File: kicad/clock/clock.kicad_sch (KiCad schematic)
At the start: 6 parts

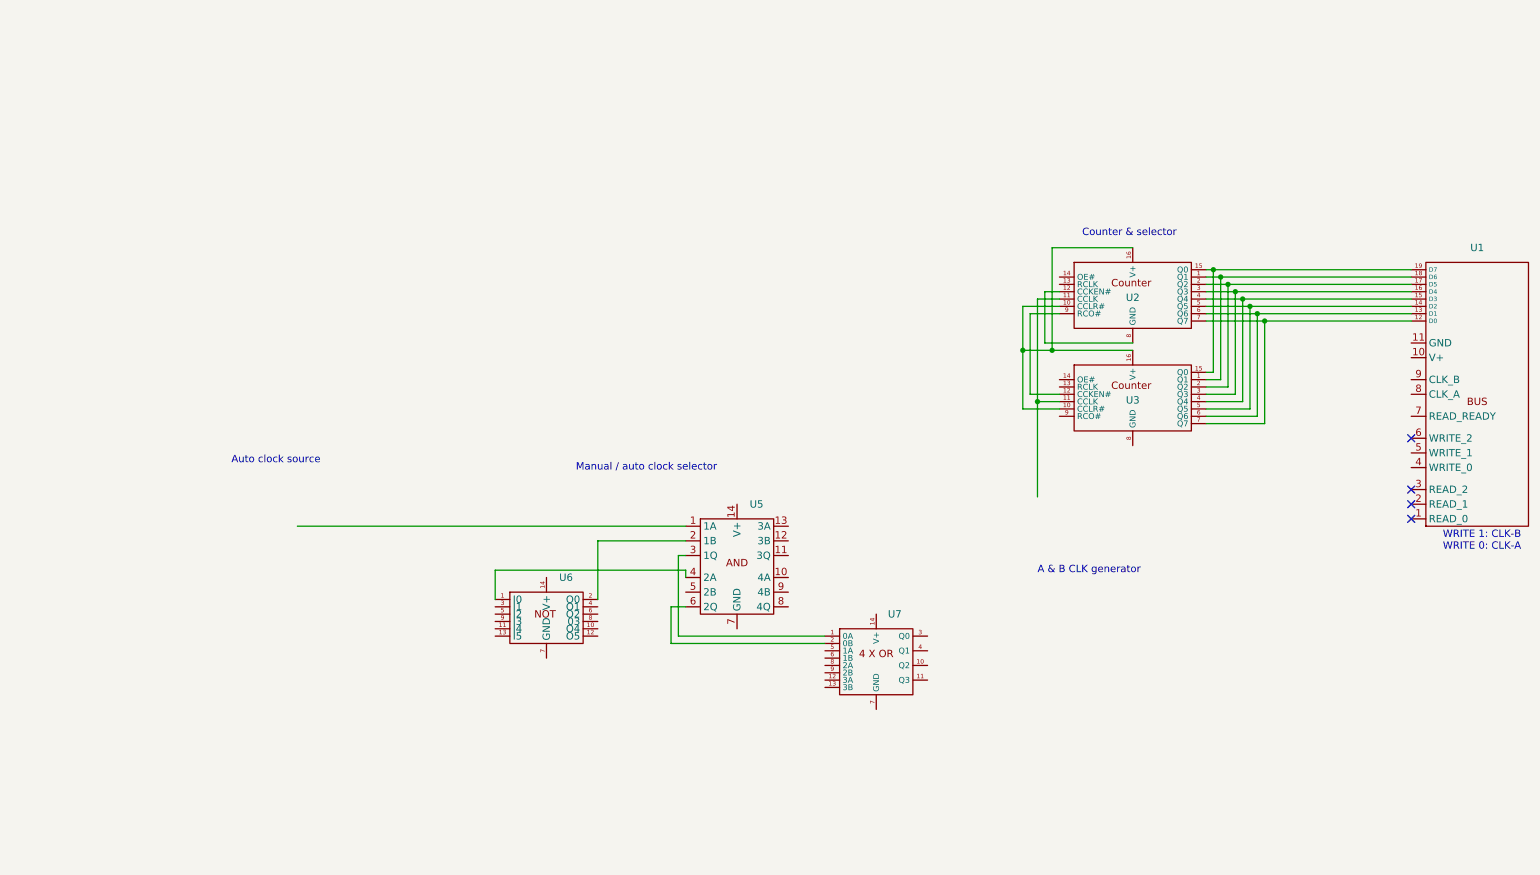
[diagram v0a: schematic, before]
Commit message: Working on clock
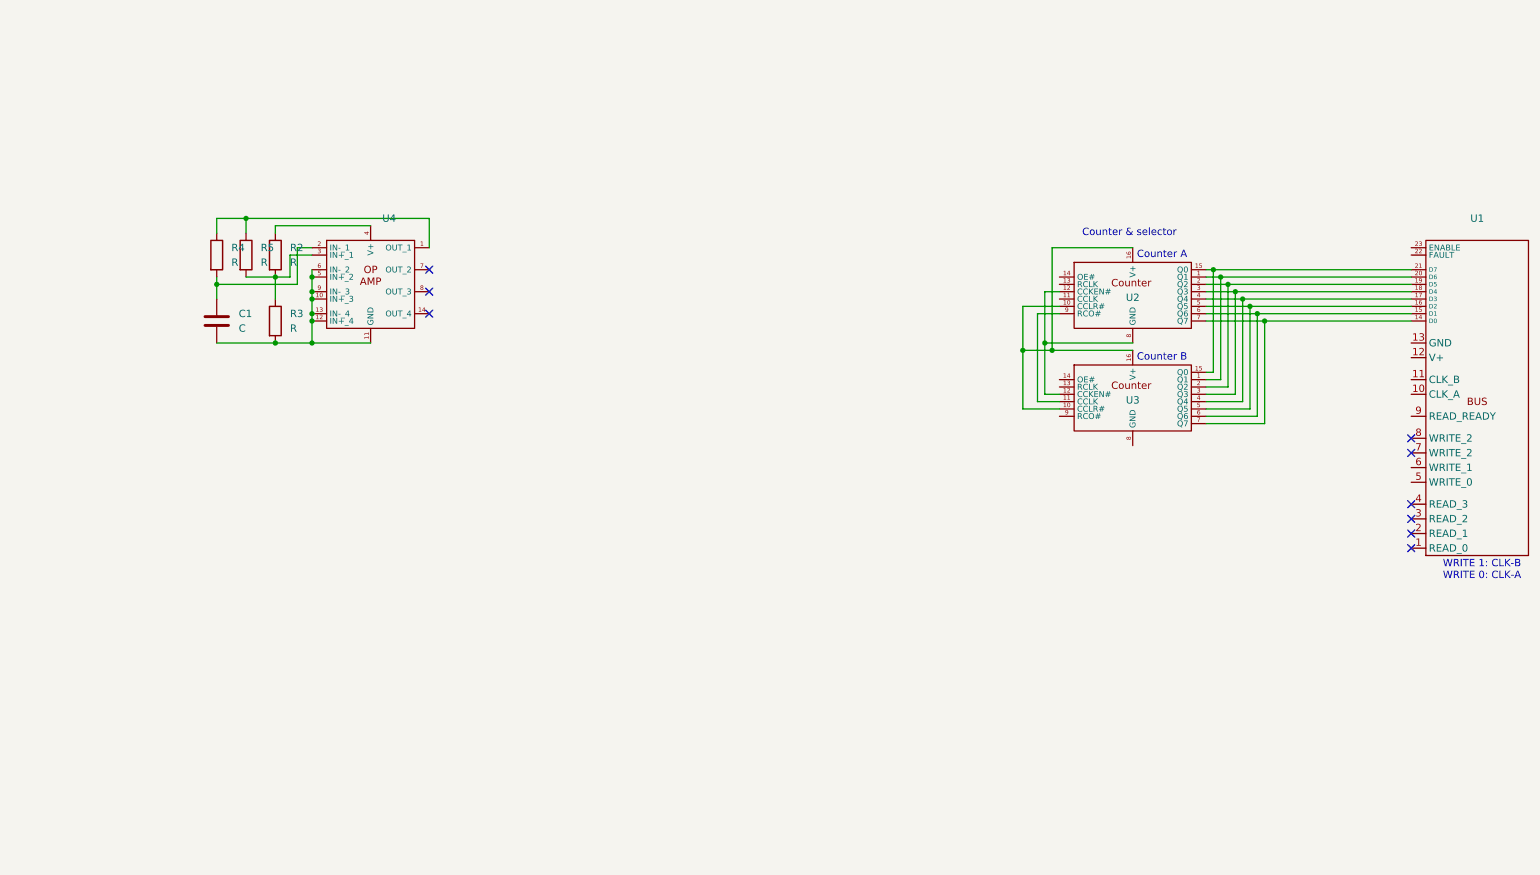
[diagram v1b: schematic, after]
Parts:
- removed U5: ~, Package_DIP:DIP-14_W7.62mm, symbol custom_symbol_lib:quad_and
- removed U6: ~, Package_DIP:DIP-14_W7.62mm, symbol custom_symbol_lib:6xNOT
- removed U7: ~, Package_DIP:DIP-14_W7.62mm, symbol custom_symbol_lib:quad_OR
- added C1: C, Capacitor_THT:C_Disc_D5.0mm_W2.5mm_P5.00mm, symbol Device:C
- added R2, R3, R4, R5: R, custom_footprint_library:0.4_pitch_resistor, symbol Device:R
- added U4: ~, Package_DIP:DIP-14_W7.62mm, symbol custom_symbol_lib:OP_AMP_quad
- U1: footprint custom_footprint_library:bus_connector -> Connector_PinHeader_2.54mm:PinHeader_1x23_P2.54mm_Vertical
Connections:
- net at U2.7 (Q7), U3.7 (Q7): now also U1.14 (D0); no longer U1.12 (D0)
- net at U2.6 (Q6), U3.6 (Q6): now also U1.15 (D1); no longer U1.13 (D1)
- net at U2.5 (Q5), U3.5 (Q5): now also U1.16 (D2); no longer U1.14 (D2)
- net at U2.4 (Q4), U3.4 (Q4): now also U1.17 (D3); no longer U1.15 (D3)
- net at U2.3 (Q3), U3.3 (Q3): now also U1.18 (D4); no longer U1.16 (D4)
- net at U2.2 (Q2), U3.2 (Q2): now also U1.19 (D5); no longer U1.17 (D5)
- net at U2.1 (Q1), U3.1 (Q1): now also U1.20 (D6); no longer U1.18 (D6)
- net at U2.15 (Q0), U3.15 (Q0): now also U1.21 (D7); no longer U1.19 (D7)
- net at U3.11 (CCLK): now also U2.9 (RCO#); no longer U2.11 (CCLK)
- net at U3.12 (CCKEN#): now also U2.12 (CCKEN#), U2.8 (GND); no longer U2.9 (RCO#)
- new net: R2.1, U4.4 (V+)
- new net: R2.2, R3.1, R5.2, U4.3 (IN+_1)
- new net: C1.1, R4.2, U4.2 (IN-_1)
- new net: C1.2, R3.2, U4.10 (IN+_3), U4.11 (GND), U4.12 (IN+_4), U4.13 (IN-_4), U4.5 (IN+_2), U4.6 (IN-_2), U4.9 (IN-_3)
- new net: R4.1, R5.1, U4.1 (OUT_1)
- no-connect marks 4 -> 9
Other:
- note added: "Counter A"
- note added: "Counter B"
- note removed: "A & B CLK generator"
- note removed: "Auto clock source"
- note removed: "Manual / auto clock selector"

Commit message: Working on clock
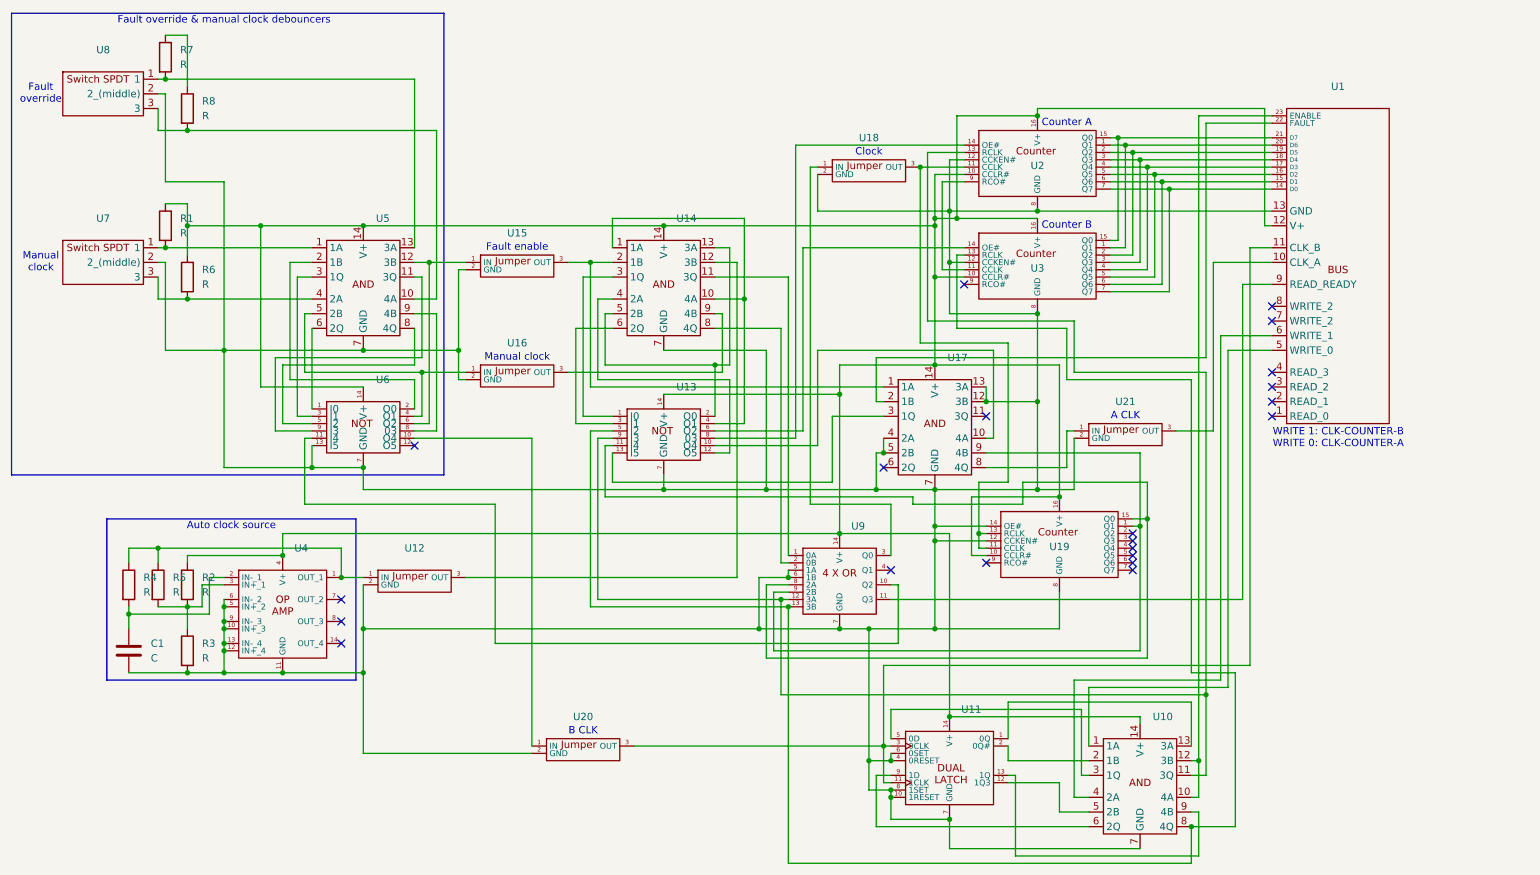
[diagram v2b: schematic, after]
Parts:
- added R1, R6, R7, R8: R, custom_footprint_library:0.4_pitch_resistor, symbol Device:R
- added U10, U14, U17, U5: ~, Package_DIP:DIP-14_W7.62mm, symbol custom_symbol_lib:quad_and
- added U11: ~, Package_DIP:DIP-14_W7.62mm, symbol custom_symbol_lib:dual_latch
- added U12, U15, U16, U18, U20, U21: ~, custom_footprint_library:jumper, symbol custom_symbol_lib:jumper
- added U13, U6: ~, Package_DIP:DIP-14_W7.62mm, symbol custom_symbol_lib:6xNOT
- added U19: ~, Package_DIP:DIP-16_W7.62mm, symbol custom_symbol_lib:8_bit_counter
- added U7, U8: ~, Connector_PinHeader_2.54mm:PinHeader_1x03_P2.54mm_Vertical, symbol custom_symbol_lib:switch_SPDT
- added U9: ~, Package_DIP:DIP-14_W7.62mm, symbol custom_symbol_lib:quad_OR
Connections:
- net at R2.1, U4.4 (V+): now also U1.12 (V+), U2.10 (CCLR#), U2.16 (V+), U3.10 (CCLR#), U3.16 (V+), R1.1, R6.1, U10.14 (V+), U11.14 (V+), U13.14 (V+), U14.14 (V+), U17.14 (V+), U19.10 (CCLR#), U19.16 (V+), U5.14 (V+), U6.14 (V+), U9.14 (V+)
- net at C1.2, R3.2, U4.10 (IN+_3)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: now also U1.13 (GND), U2.12 (CCKEN#), U2.8 (GND), U3.12 (CCKEN#), U3.8 (GND), U10.7 (GND), U11.10 (1RESET), U11.4 (0RESET), U11.6 (0SET), U11.7 (GND), U11.8 (1SET), U12.2 (GND), U13.7 (GND), U14.7 (GND), U15.2 (GND), U16.2 (GND), U17.12 (3B), U17.13 (3A), U17.4 (2A), U17.5 (2B), U17.7 (GND), U18.2 (GND), U19.12 (CCKEN#), U19.14 (OE#), U19.8 (GND), U20.2 (GND), U21.2 (GND), U5.7 (GND), U6.13 (I5), U6.7 (GND), U7.2 (2_(middle)), U8.2 (2_(middle)), U9.5 (1A), U9.6 (1B), U9.7 (GND)
- net at R4.1, R5.1, U4.1 (OUT_1): now also U12.1 (IN)
- net at U1.10 (CLK_A): now also U21.3 (OUT)
- net at U1.11 (CLK_B): now also U11.11 (1CLK), U11.3 (0CLK), U20.3 (OUT)
- net at U1.22 (FAULT): now also U17.2 (1B)
- net at U1.23 (ENABLE): now also U10.10 (4A), U10.12 (3B)
- net at U1.5 (WRITE_0): now also U10.1 (1A)
- net at U1.6 (WRITE_1): now also U10.4 (2A)
- net at U1.9 (READ_READY): now also U9.11 (Q3)
- net at U3.13 (RCLK): now also U10.8 (4Q), U13.5 (I2), U9.13 (3B)
- net at U3.14 (OE#): now also U13.6 (O2)
- net at U2.11 (CCLK): now also U18.3 (OUT), U19.11 (CCLK), U19.13 (RCLK)
- net at U2.13 (RCLK): now also U10.11 (3Q), U13.9 (I3), U9.12 (3A)
- net at U2.14 (OE#): now also U13.8 (03)
- new net: R1.2, U5.1 (1A), U7.1
- new net: R6.2, U5.4 (2A), U7.3
- new net: U17.9 (4B), U19.1 (Q1), U9.9 (2B)
- new net: U13.11 (I4), U19.15 (Q0), U9.8 (2A)
- new net: U12.3 (OUT), U14.12 (3B)
- new net: U20.1 (IN), U6.10 (O4)
- new net: U16.1 (IN), U5.5 (2B), U6.4 (O1)
- new net: U14.9 (4B), U16.3 (OUT)
- new net: U14.11 (3Q), U9.1 (0A)
- new net: U6.11 (I4), U9.10 (Q2)
- new net: U14.8 (4Q), U9.2 (0B)
- new net: U18.1 (IN), U9.3 (Q0)
- new net: U10.13 (3A), U11.1 (0Q)
- new net: U10.5 (2B), U11.12 (1Q3)
- new net: U10.9 (4B), U11.13 (1Q)
- new net: U10.2 (1B), U11.2 (0Q#)
- new net: U10.3 (1Q), U11.5 (0D)
- new net: U10.6 (2Q), U11.9 (1D)
- new net: U14.2 (1B), U15.3 (OUT), U17.1 (1A)
- new net: U13.10 (O4), U17.10 (4A)
- new net: U13.13 (I5), U17.3 (1Q)
- new net: U17.8 (4Q), U21.1 (IN)
- new net: R7.1, R8.1
- new net: R7.2, U5.13 (3A), U8.1
- new net: U13.4 (O1), U14.1 (1A), U14.10 (4A)
- new net: U13.2 (O0), U14.13 (3A), U14.5 (2B)
- new net: U13.1 (I0), U14.3 (1Q)
- new net: U13.12 (O5), U14.4 (2A)
- new net: U13.3 (I1), U14.6 (2Q)
- new net: U15.1 (IN), U5.12 (3B), U6.6 (O2)
- new net: R8.2, U5.10 (4A), U8.3
- new net: U5.6 (2Q), U6.1 (I0)
- new net: U5.2 (1B), U6.2 (O0)
- new net: U5.3 (1Q), U6.3 (I1)
- new net: U5.8 (4Q), U6.5 (I2)
- new net: U5.9 (4B), U6.8 (03)
- new net: U5.11 (3Q), U6.9 (I3)
- no-connect marks 9 -> 21
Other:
- note added: "A CLK"
- note added: "Auto clock source"
- note added: "B CLK"
- note added: "Clock"
- note added: "Fault enable"
- note added: "Fault override"
- note added: "Fault override & manual clock debouncers"
- note added: "Manual clock"
- note added: "WRITE 1: CLK-COUNTER-B WRITE 0: CLK-COUNTER-A"
- note removed: "Counter & selector"
- note removed: "WRITE 1: CLK-B WRITE 0: CLK-A"
- moved on the sheet: C1, R2, R3, R4, R5, U1, U2, U3, U4
